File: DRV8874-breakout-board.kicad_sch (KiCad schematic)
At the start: 16 parts, among them J102 Conn_01x02_Pin, J104 Conn_01x06_Pin, J105 PMODE, J305 M0_CONN

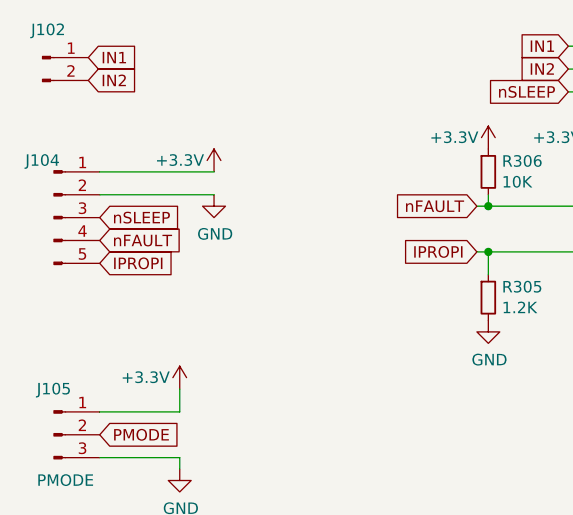
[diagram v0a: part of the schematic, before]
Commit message: Additional changes
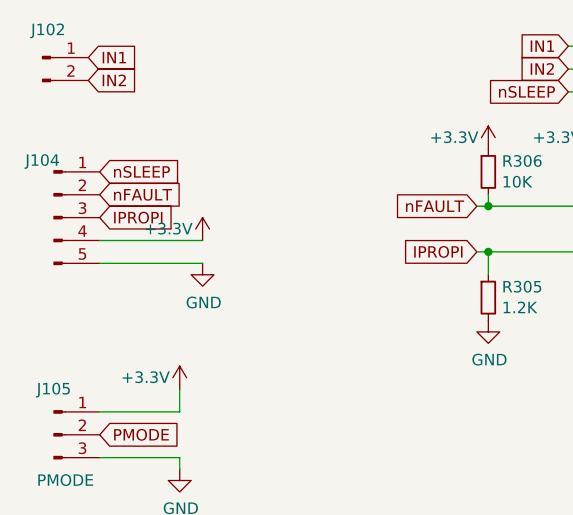
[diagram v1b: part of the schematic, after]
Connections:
- net +3V3: now also J104.4 (Pin_4); no longer J104.1 (Pin_1)
- net GND: now also J104.5 (Pin_5); no longer J104.2 (Pin_2)
- net IPROPI: now also J104.3 (Pin_3); no longer J104.5 (Pin_5)
- net nFAULT: now also J104.2 (Pin_2); no longer J104.4 (Pin_4)
- net nSLEEP: now also J104.1 (Pin_1); no longer J104.3 (Pin_3)
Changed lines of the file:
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@@
-    (stroke (width 0) (type default))
-  )
-  (wire (pts (xy 71.12 91.44) (xy 83.82 91.44))
     (stroke (width 0) (type default))
   )
@@
     (stroke (width 0) (type default))
   )
+  (wire (pts (xy 71.12 96.52) (xy 82.55 96.52))
+    (stroke (width 0) (type default))
+  )
   (wire (pts (xy 154.94 87.63) (xy 158.75 87.63))
     (stroke (width 0) (type default))
@@
     (stroke (width 0) (type default))
   )
-  (wire (pts (xy 71.12 88.9) (xy 83.82 88.9))
-    (stroke (width 0) (type default))
-  )
   (wire (pts (xy 170.18 105.41) (xy 170.18 113.03))
     (stroke (width 0) (type default))
   )
   (wire (pts (xy 158.75 81.28) (xy 176.53 81.28))
+    (stroke (width 0) (type default))
+  )
+  (wire (pts (xy 71.12 99.06) (xy 82.55 99.06))
     (stroke (width 0) (type default))
   )
@@
     )
   )
-  (global_label "nFAULT" (shape input) (at 71.12 96.52 0)
+  (global_label "nFAULT" (shape input) (at 71.12 91.44 0)
     (effects (font (size 1.27 1.27)) (justify left))
-    (property "Intersheetrefs" "${INTERSHEET_REFS}" (at 71.12 96.52 0)
+    (property "Intersheetrefs" "${INTERSHEET_REFS}" (at 71.12 91.44 0)
       (effects (font (size 1.27 1.27)) hide)
     )
@@
     )
   )
-  (global_label "IPROPI" (shape input) (at 71.12 99.06 0)
+  (global_label "IPROPI" (shape input) (at 71.12 93.98 0)
     (effects (font (size 1.27 1.27)) (justify left))
-    (property "Intersheetrefs" "${INTERSHEET_REFS}" (at 71.12 99.06 0)
+    (property "Intersheetrefs" "${INTERSHEET_REFS}" (at 71.12 93.98 0)
       (effects (font (size 1.27 1.27)) hide)
     )
@@
     )
   )
-  (global_label "nSLEEP" (shape input) (at 71.12 93.98 0)
+  (global_label "nSLEEP" (shape input) (at 71.12 88.9 0)
     (effects (font (size 1.27 1.27)) (justify left))
-    (property "Intersheetrefs" "${INTERSHEET_REFS}" (at 71.12 93.98 0)
+    (property "Intersheetrefs" "${INTERSHEET_REFS}" (at 71.12 88.9 0)
       (effects (font (size 1.27 1.27)) hide)
     )
@@
     )
   )
-  (symbol (lib_id "power:GND") (at 83.82 91.44 0) (unit 1)
-    (in_bom yes) (on_board yes) (dnp no)
-    (property "Reference" "#PWR0323" (at 83.82 97.79 0)
-      (effects (font (size 1.27 1.27)) hide)
-    )
-    (property "Value" "GND" (at 83.947 95.8342 0)
-      (effects (font (size 1.27 1.27)))
-    )
-    (property "Footprint" "" (at 83.82 91.44 0)
-      (effects (font (size 1.27 1.27)) hide)
-    )
-    (property "Datasheet" "" (at 83.82 91.44 0)
+  (symbol (lib_id "power:GND") (at 82.55 99.06 0) (unit 1)
+    (in_bom yes) (on_board yes) (dnp no)
+    (property "Reference" "#PWR0323" (at 82.55 105.41 0)
+      (effects (font (size 1.27 1.27)) hide)
+    )
+    (property "Value" "GND" (at 82.677 103.4542 0)
+      (effects (font (size 1.27 1.27)))
+    )
+    (property "Footprint" "" (at 82.55 99.06 0)
+      (effects (font (size 1.27 1.27)) hide)
+    )
+    (property "Datasheet" "" (at 82.55 99.06 0)
       (effects (font (size 1.27 1.27)) hide)
     )
@@
     )
   )
-  (symbol (lib_id "smart_motor_controller-rescue:+3.3V-power") (at 83.82 88.9 0) (unit 1)
-    (in_bom yes) (on_board yes) (dnp no)
-    (property "Reference" "#PWR0324" (at 83.82 92.71 0)
-      (effects (font (size 1.27 1.27)) hide)
-    )
-    (property "Value" "+3.3V" (at 80.01 87.63 0)
-      (effects (font (size 1.27 1.27)))
-    )
-    (property "Footprint" "" (at 83.82 88.9 0)
-      (effects (font (size 1.27 1.27)) hide)
-    )
-    (property "Datasheet" "" (at 83.82 88.9 0)
-      (effects (font (size 1.27 1.27)) hide)
-    )
+  (symbol (lib_id "smart_motor_controller-rescue:+3.3V-power") (at 82.55 96.52 0) (unit 1)
+    (in_bom yes) (on_board yes) (dnp no)
+    (property "Reference" "#PWR0324" (at 82.55 100.33 0)
+      (effects (font (size 1.27 1.27)) hide)
+    )
+    (property "Value" "+3.3V" (at 78.74 95.25 0)
+      (effects (font (size 1.27 1.27)))
+    )
+    (property "Footprint" "" (at 82.55 96.52 0)
+      (effects (font (size 1.27 1.27)) hide)
+    )
+    (property "Datasheet" "" (at 82.55 96.52 0)
+      (effects (font (size 1.27 1.27)) hide)
+    )
